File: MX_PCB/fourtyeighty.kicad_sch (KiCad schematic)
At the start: 148 parts, among them J1 USB_C_Receptacle_USB2.0, SW1 RotaryEncoder_Switch, U1 XC6206PxxxMR, U2 SRV05-4, U3 W25Q128JVS, U4 RP2040TR7, Y1 Crystal_GND24_Small

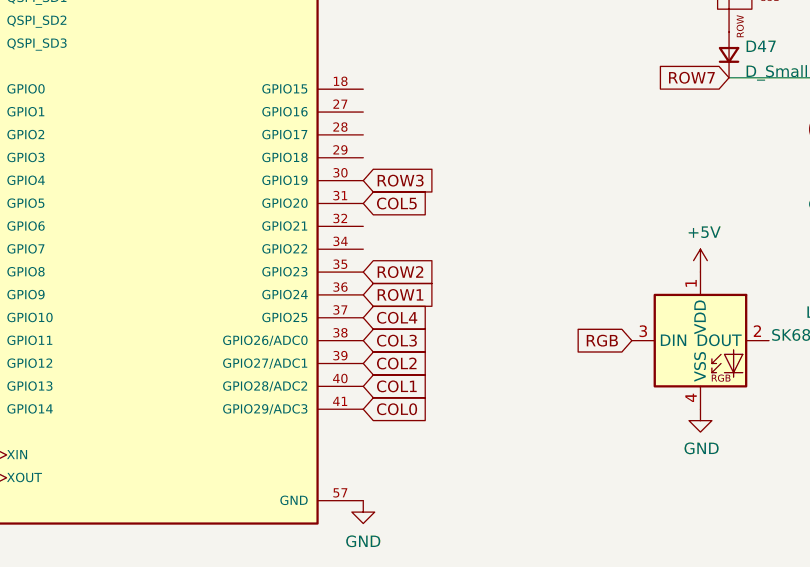
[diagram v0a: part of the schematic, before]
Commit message: Completed MX PCB
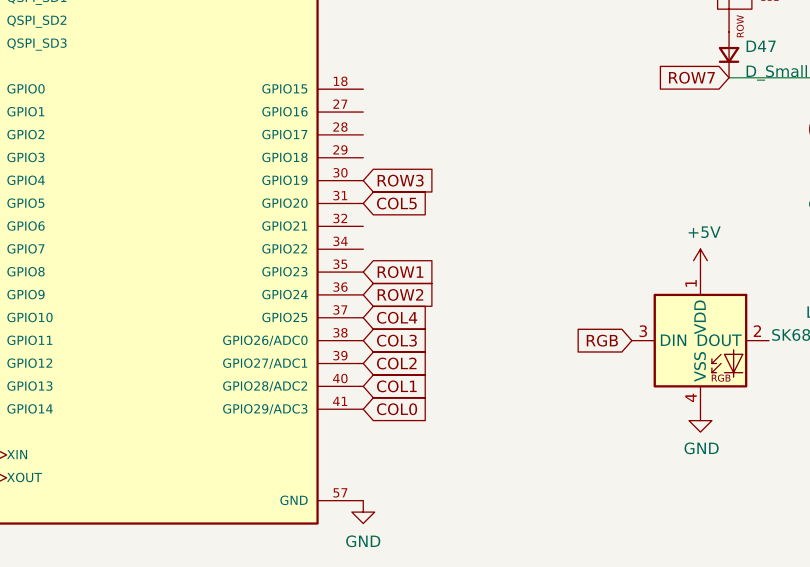
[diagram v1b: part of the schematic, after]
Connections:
- net ROW1: now also U4.35 (GPIO23); no longer U4.36 (GPIO24)
- net ROW2: now also U4.36 (GPIO24); no longer U4.35 (GPIO23)
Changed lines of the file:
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@@
     )
   )
-  (global_label "ROW1" (shape input) (at 74.93 161.29 0) (fields_autoplaced)
+  (global_label "ROW1" (shape input) (at 74.93 158.75 0) (fields_autoplaced)
     (effects (font (size 1.27 1.27)) (justify left))
-    (property "Intersheetrefs" "${INTERSHEET_REFS}" (at 83.0972 161.29 0)
+    (property "Intersheetrefs" "${INTERSHEET_REFS}" (at 83.0972 158.75 0)
       (effects (font (size 1.27 1.27)) (justify left) hide)
     )
@@
     )
   )
-  (global_label "ROW2" (shape input) (at 74.93 158.75 0) (fields_autoplaced)
+  (global_label "ROW2" (shape input) (at 74.93 161.29 0) (fields_autoplaced)
     (effects (font (size 1.27 1.27)) (justify left))
-    (property "Intersheetrefs" "${INTERSHEET_REFS}" (at 83.0972 158.75 0)
+    (property "Intersheetrefs" "${INTERSHEET_REFS}" (at 83.0972 161.29 0)
       (effects (font (size 1.27 1.27)) (justify left) hide)
     )
